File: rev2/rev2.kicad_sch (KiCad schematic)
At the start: 4 parts, among them U1 STM32F030RCTx, Y1 16mhz

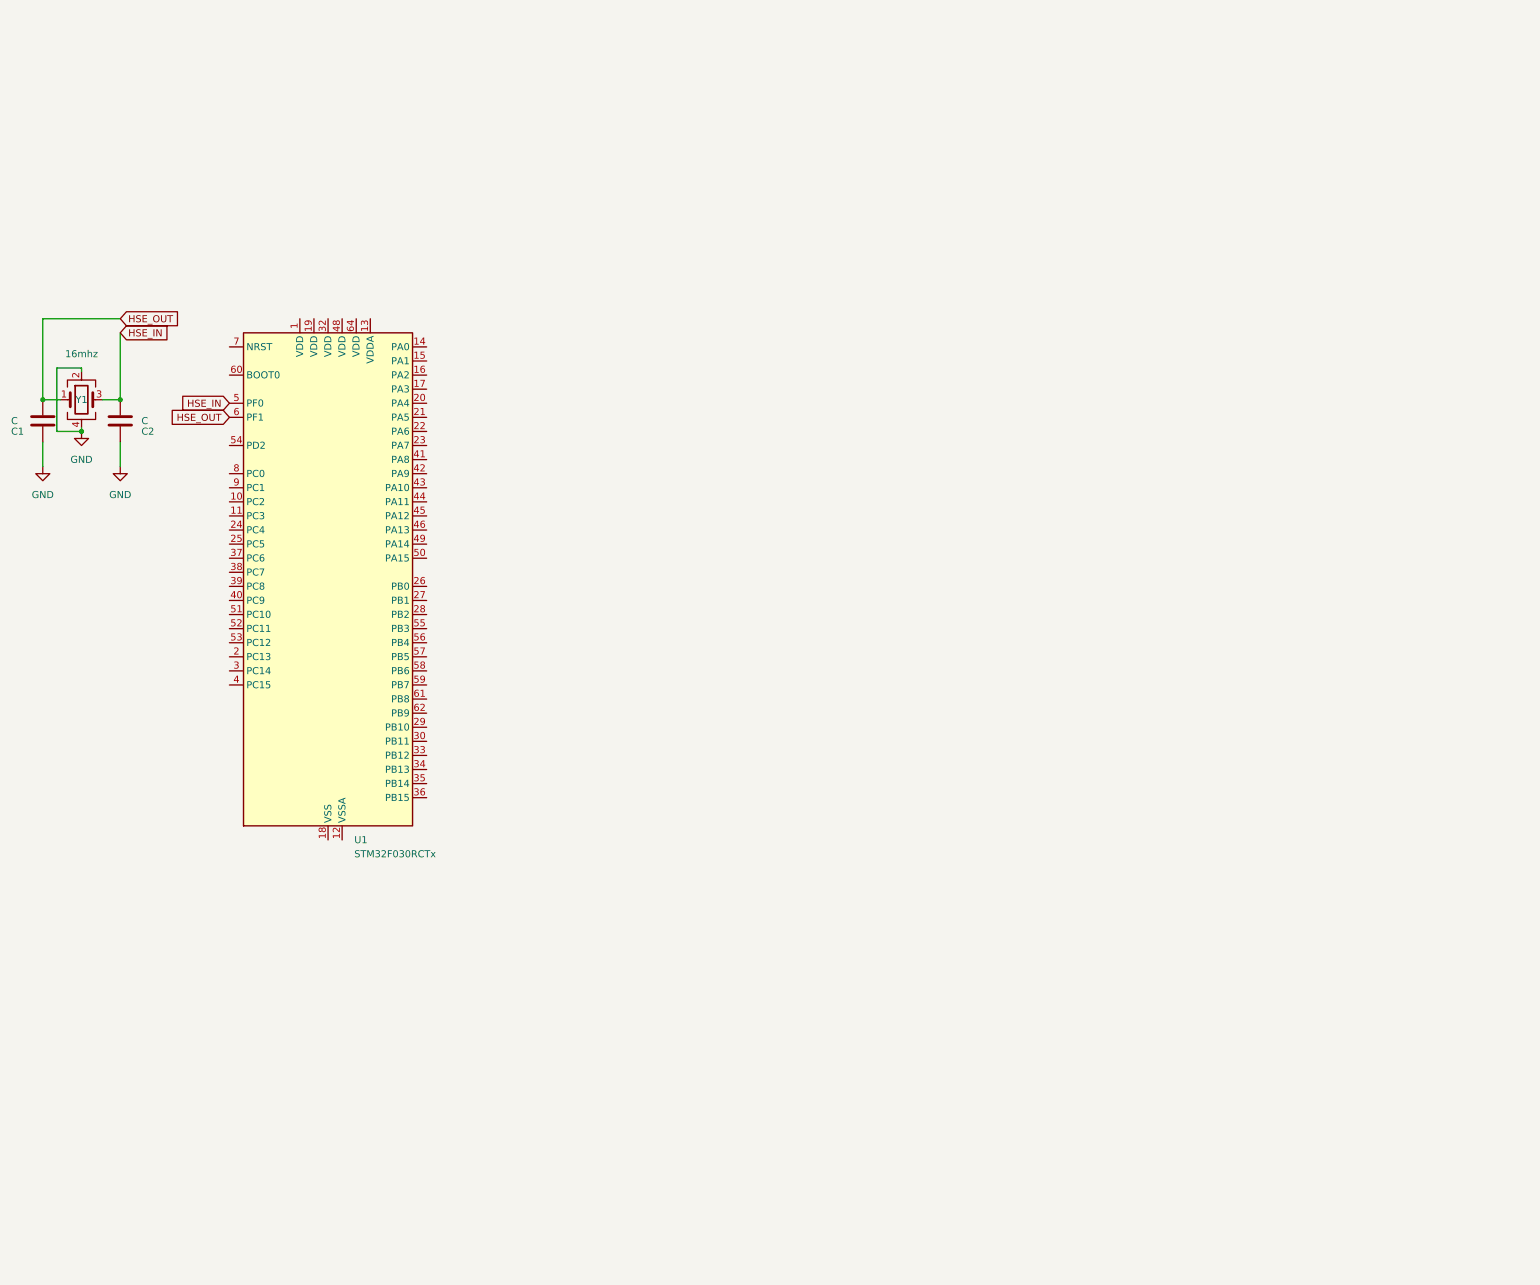
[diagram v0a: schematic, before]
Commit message: added changes to the rev 2 board
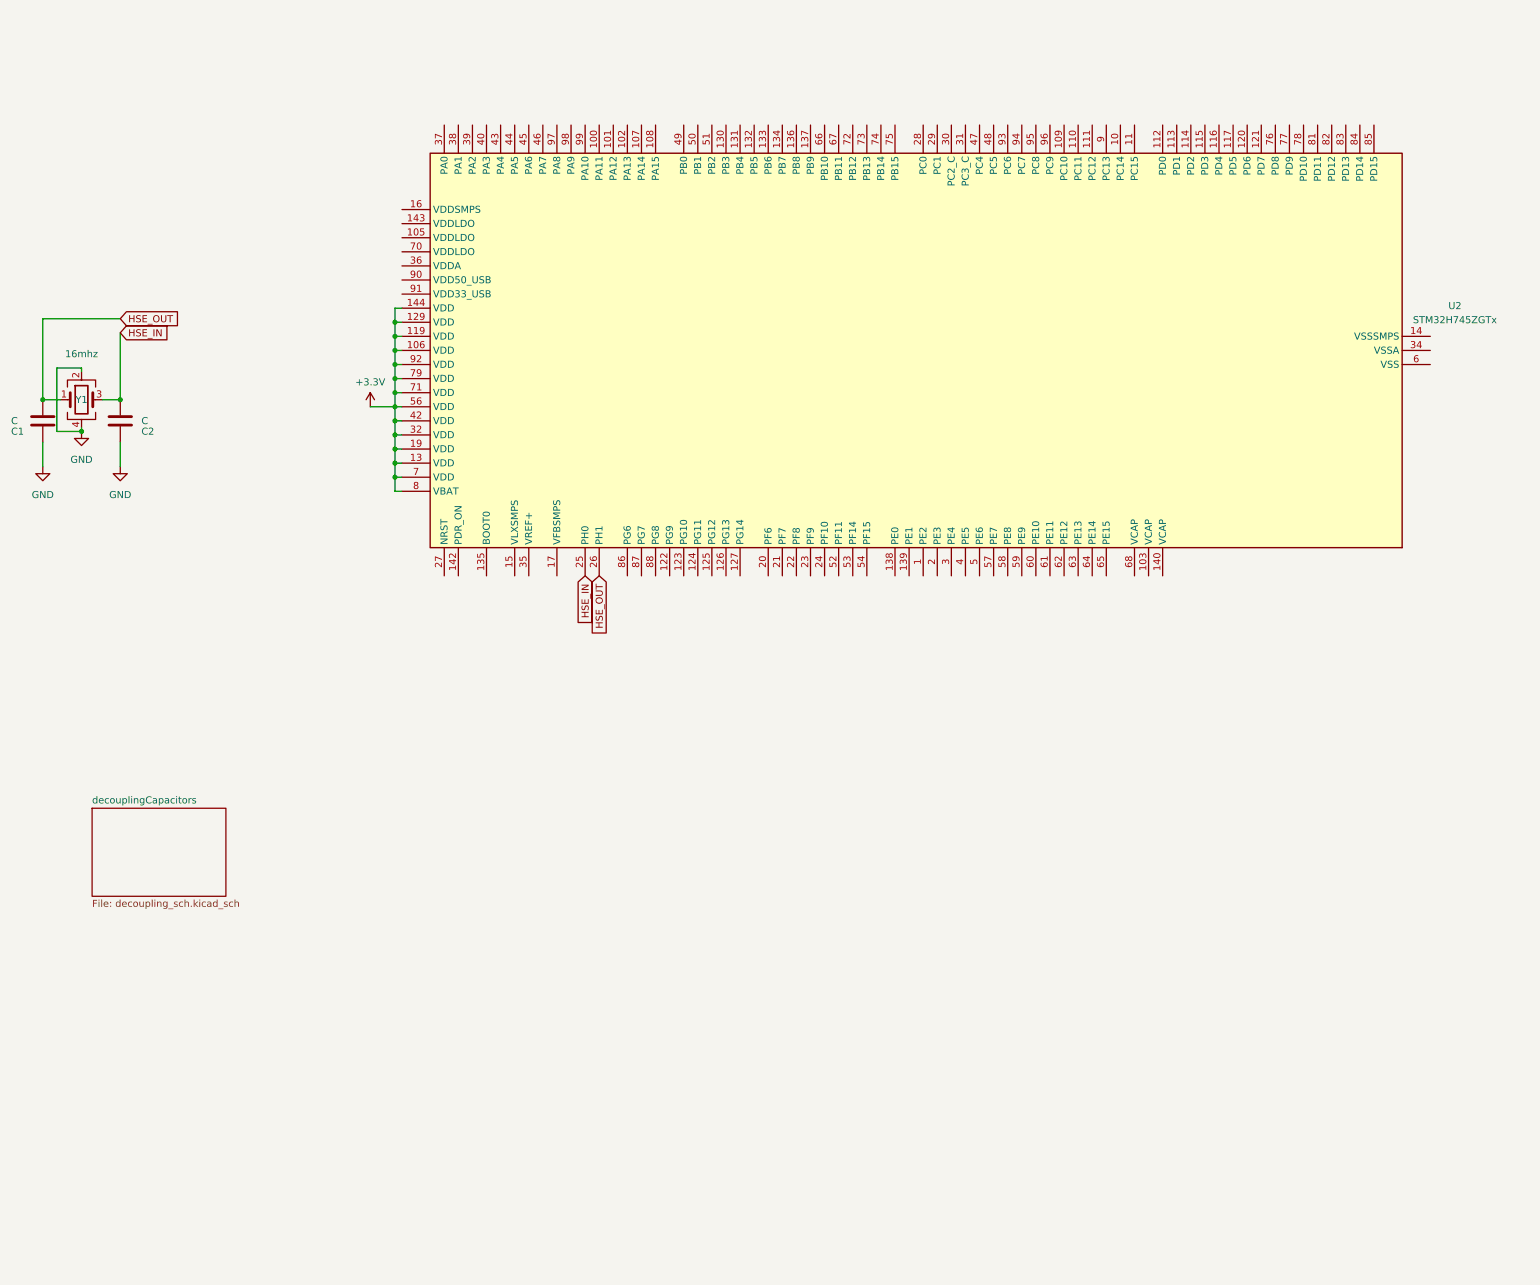
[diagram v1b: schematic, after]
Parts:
- removed U1: STM32F030RCTx, Package_QFP:LQFP-64_10x10mm_P0.5mm, symbol MCU_ST_STM32F0:STM32F030RCTx
- added U2: STM32H745ZGTx, Package_QFP:LQFP-144_20x20mm_P0.5mm, symbol MCU_ST_STM32H7:STM32H745ZGTx
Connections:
- net HSE_IN: now also U2.25 (PH0)
- net HSE_OUT: now also U2.26 (PH1)
- new net: U2.104 (VSS), U2.118 (VSS), U2.12 (VSS), U2.128 (VSS), U2.141 (VSS), U2.18 (VSS), U2.33 (VSS), U2.41 (VSS), U2.55 (VSS), U2.6 (VSS), U2.69 (VSS), U2.80 (VSS), U2.89 (VSS)
- new net +3.3V: U2.106 (VDD), U2.119 (VDD), U2.129 (VDD), U2.13 (VDD), U2.144 (VDD), U2.19 (VDD), U2.32 (VDD), U2.42 (VDD), U2.56 (VDD), U2.7 (VDD), U2.71 (VDD), U2.79 (VDD), U2.8 (VBAT), U2.92 (VDD)
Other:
- added sheet decouplingCapacitors (decoupling_sch.kicad_sch)

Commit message: something
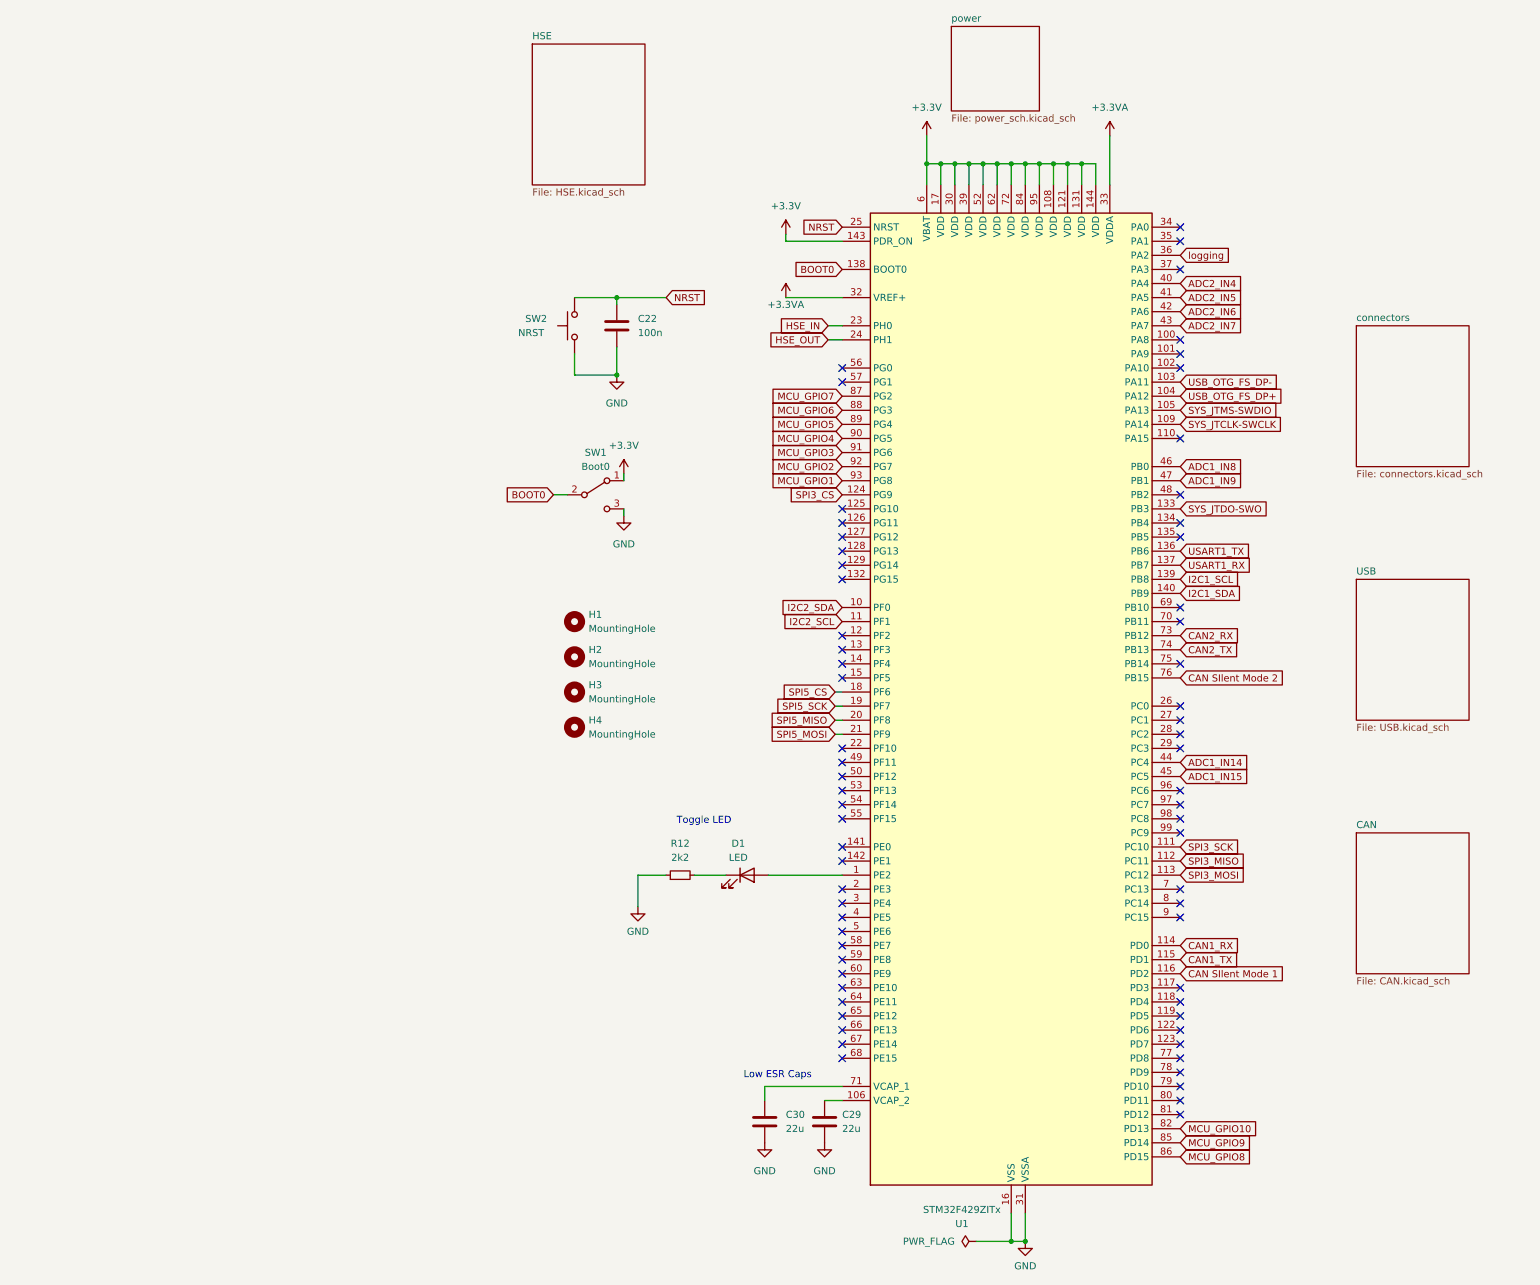
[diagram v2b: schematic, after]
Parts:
- removed C1, C2: C, symbol Device:C
- removed U2: STM32H745ZGTx, Package_QFP:LQFP-144_20x20mm_P0.5mm, symbol MCU_ST_STM32H7:STM32H745ZGTx
- removed Y1: 16mhz, symbol Device:Crystal_GND24
- added C22: 100n, Capacitor_SMD:C_0603_1608Metric_Pad1.08x0.95mm_HandSolder, symbol Device:C
- added C29, C30: 22u, Capacitor_SMD:C_0603_1608Metric_Pad1.08x0.95mm_HandSolder, symbol Device:C
- added D1: LED, LED_SMD:LED_0603_1608Metric_Pad1.05x0.95mm_HandSolder, symbol Device:LED
- added H1, H2, H3, H4: MountingHole, MountingHole:MountingHole_4.3mm_M4_Pad_Via, symbol Mechanical:MountingHole
- added R12: 2k2, Resistor_SMD:R_0603_1608Metric_Pad0.98x0.95mm_HandSolder, symbol Device:R_Small
- added SW1: Boot0, Button_Switch_SMD:SW_SPDT_CK-JS102011SAQN, symbol Switch:SW_SPDT
- added SW2: NRST, Button_Switch_SMD:SW_SPST_PTS645, symbol Switch:SW_Push
- added U1: STM32F429ZITx, Package_QFP:LQFP-144_20x20mm_P0.5mm, symbol MCU_ST_STM32F4:STM32F429ZITx
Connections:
- net +3.3V: now also SW1.1 (A), U1.108 (VDD), U1.121 (VDD), U1.131 (VDD), U1.143 (PDR_ON), U1.144 (VDD), U1.17 (VDD), U1.30 (VDD), U1.39 (VDD), U1.52 (VDD), U1.6 (VBAT), U1.62 (VDD), U1.72 (VDD), U1.84 (VDD), U1.95 (VDD)
- net GND: now also C22.2, C29.2, C30.2, R12.1, SW1.3 (C), SW2.1, U1.107 (VSS), U1.120 (VSS), U1.130 (VSS), U1.16 (VSS), U1.31 (VSSA), U1.38 (VSS), U1.51 (VSS), U1.61 (VSS), U1.83 (VSS), U1.94 (VSS)
- net HSE_OUT: now also U1.24 (PH1)
- new net: C30.1, U1.71 (VCAP_1)
- new net: D1.2 (A), U1.1 (PE2)
- new net: C29.1, U1.106 (VCAP_2)
- new net: D1.1 (K), R12.2
- new net +3.3VA: U1.32 (VREF+), U1.33 (VDDA)
- new net ADC1_IN14: U1.44 (PC4)
- new net ADC1_IN15: U1.45 (PC5)
- new net ADC1_IN8: U1.46 (PB0)
- new net ADC1_IN9: U1.47 (PB1)
- new net ADC2_IN4: U1.40 (PA4)
- new net ADC2_IN5: U1.41 (PA5)
- new net ADC2_IN6: U1.42 (PA6)
- new net ADC2_IN7: U1.43 (PA7)
- new net BOOT0: SW1.2 (B), U1.138 (BOOT0)
- new net CAN SIlent Mode 1: U1.116 (PD2)
- new net CAN SIlent Mode 2: U1.76 (PB15)
- new net CAN1_RX: U1.114 (PD0)
- new net CAN1_TX: U1.115 (PD1)
- new net CAN2_RX: U1.73 (PB12)
- new net CAN2_TX: U1.74 (PB13)
- new net HSE_IN  : U1.23 (PH0)
- new net I2C1_SCL: U1.139 (PB8)
- new net I2C1_SDA: U1.140 (PB9)
- new net I2C2_SCL: U1.11 (PF1)
- new net I2C2_SDA: U1.10 (PF0)
- new net MCU_GPIO1: U1.93 (PG8)
- new net MCU_GPIO10: U1.82 (PD13)
- new net MCU_GPIO2: U1.92 (PG7)
- new net MCU_GPIO3: U1.91 (PG6)
- new net MCU_GPIO4: U1.90 (PG5)
- new net MCU_GPIO5: U1.89 (PG4)
- new net MCU_GPIO6: U1.88 (PG3)
- new net MCU_GPIO7: U1.87 (PG2)
- new net MCU_GPIO8: U1.86 (PD15)
- new net MCU_GPIO9: U1.85 (PD14)
- new net NRST: C22.1, SW2.2, U1.25 (NRST)
- new net SPI3_CS  : U1.124 (PG9)
- new net SPI3_MISO: U1.112 (PC11)
- new net SPI3_MOSI: U1.113 (PC12)
- new net SPI3_SCK: U1.111 (PC10)
- new net SPI5_CS  : U1.18 (PF6)
- new net SPI5_MISO: U1.20 (PF8)
- new net SPI5_MOSI: U1.21 (PF9)
- new net SPI5_SCK : U1.19 (PF7)
- new net SYS_JTCLK-SWCLK: U1.109 (PA14)
- new net SYS_JTDO-SWO: U1.133 (PB3)
- new net SYS_JTMS-SWDIO: U1.105 (PA13)
- new net USART1_RX: U1.137 (PB7)
- new net USART1_TX: U1.136 (PB6)
- new net USB_OTG_FS_DP+: U1.104 (PA12)
- new net USB_OTG_FS_DP-: U1.103 (PA11)
- new net logging: U1.36 (PA2)
- no-connect marks 0 -> 67
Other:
- removed sheet decouplingCapacitors
- added sheet CAN (CAN.kicad_sch)
- added sheet HSE (HSE.kicad_sch)
- added sheet USB (USB.kicad_sch)
- added sheet connectors (connectors.kicad_sch)
- added sheet power (power_sch.kicad_sch)
- note added: "Low ESR Caps"
- note added: "Toggle LED"
